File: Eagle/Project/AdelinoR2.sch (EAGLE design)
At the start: 68 parts, among them J1 DC-044-A, J2 YELLOW-8P-2.54, J3 YELLOW-6P-2.54, J4 YELLOW-8P-2.54, J5 YELLOW-8P-2.54, J6 4P-2.0, J7 YELLOW-2X3P-2.54, J8 4P-2.0, Q1 NCE3407A, Q2 CJ2305, SW1 TS-1101F, U1 MP1496DJ-SOT23-8, U2 CJT1117-3.3-SOT223, U3 ESP-12F / OPL: 317060163 / SM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, U4 ATMEGA32U4-MUR-QFN44, U5 74VHC125MTCX-TSSOP14, U6 ATMEGA32U4-TQFP44, X1 306010049_XTAL_16MHZ-3225_4P

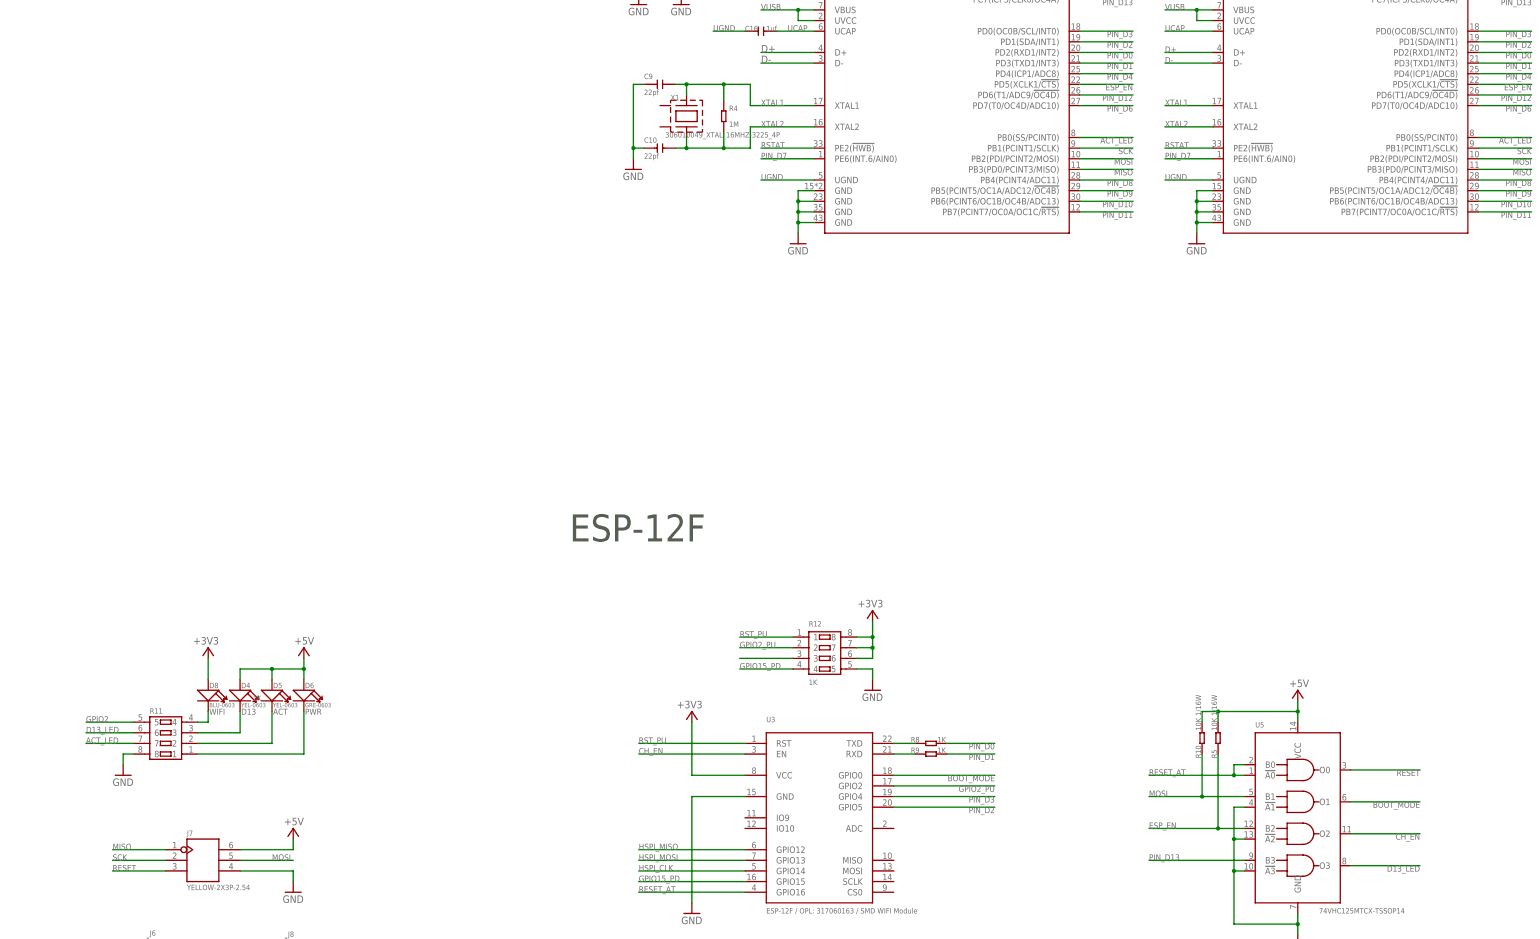
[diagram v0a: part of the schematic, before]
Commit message: Wip.
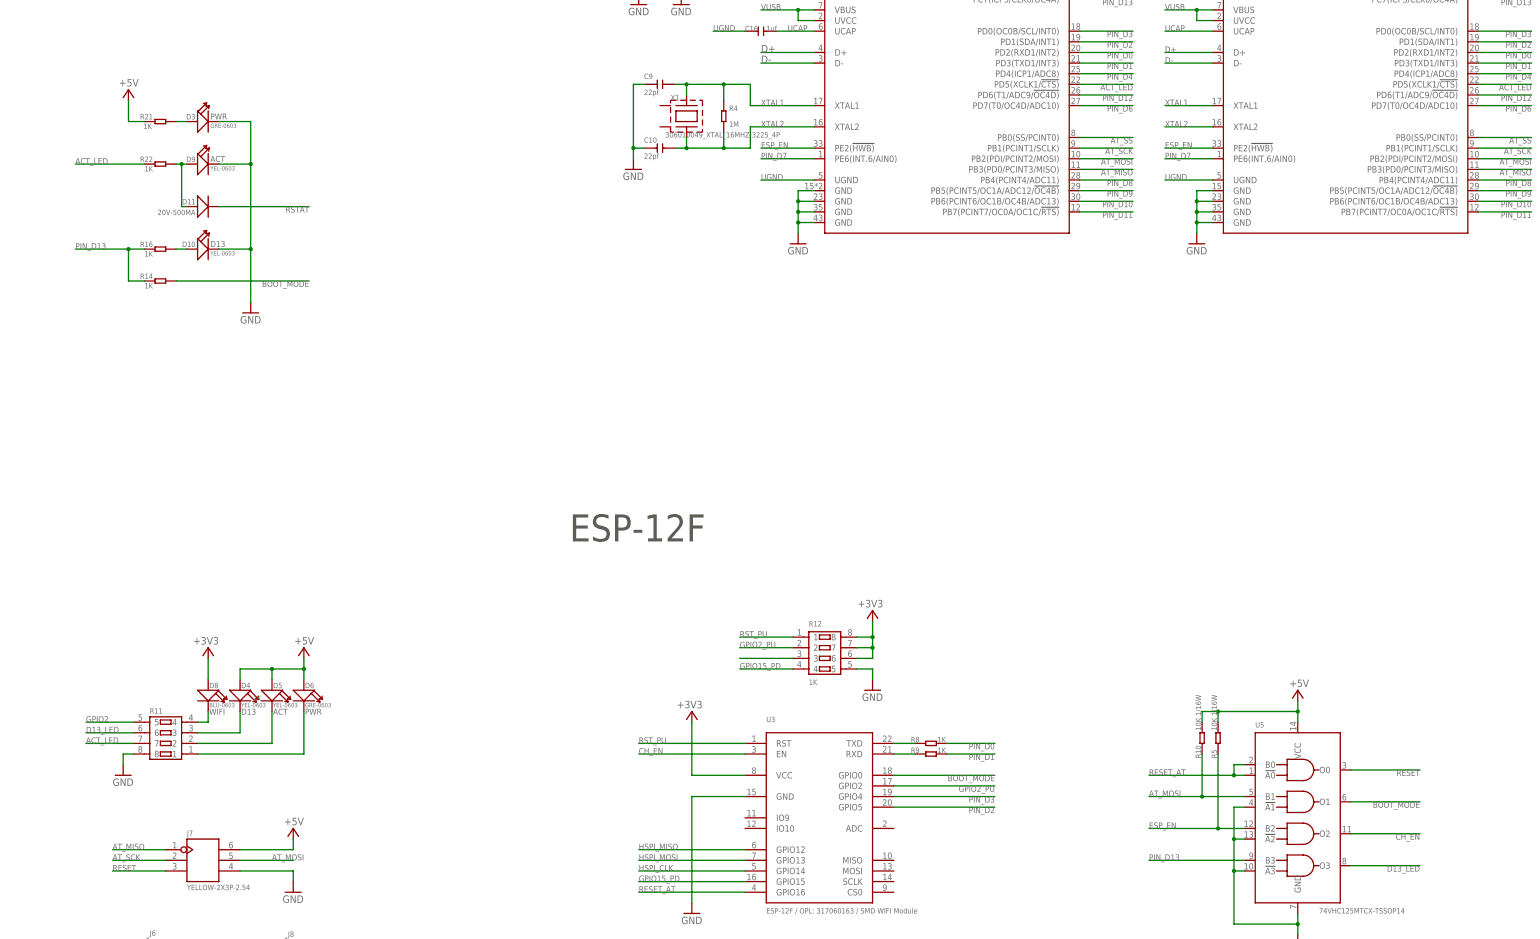
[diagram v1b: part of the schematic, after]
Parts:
- added D10, D9: YEL-0603, Seeed-LED:SMD-LED-CLEAR-YELLOW(0603)
- added D11: 20V-500MA, Seeed-Diode:SMD-DIODE-SCHOTTKY-20V-500MA(SOD-123)P
- added D3: GRE-0603, Seeed-LED:SMD-LED-CLEAR-GREEN(0603)
- added R14, R16, R21, R22: 1K, Seeed-Resistor:SMD-RES-1K-5%-1/16W(0402)
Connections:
- net MISO renamed AT_MISO
- net MOSI renamed AT_MOSI
- net SCK renamed AT_SCK
- new net AT_SS: U4.PB0(SS/PCINT0), U6.PB0(SS/PCINT0)
- new net N$10: D10.+, R16.2
- new net N$4: D3.+, R21.2
- new net N$7: D11.+, D9.+, R22.2
- net +5V: now also R21.1
- net ACT_LED: now also R22.1, U4.PD5(XCLK1/!CTS), U6.PD5(XCLK1/!CTS); no longer U4.PB0(SS/PCINT0), U6.PB0(SS/PCINT0)
- net BOOT_MODE: now also R14.2
- net ESP_EN: now also U4.PE2(!HWB), U6.PE2(!HWB); no longer U4.PD5(XCLK1/!CTS), U6.PD5(XCLK1/!CTS)
- net GND: now also D10.-, D3.-, D9.-
- net PIN_D13: now also R14.1, R16.1
- net RSTAT: now also D11.-; no longer U4.PE2(!HWB), U6.PE2(!HWB)
